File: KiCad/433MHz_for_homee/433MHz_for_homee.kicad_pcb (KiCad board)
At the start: 2 copper layers, 90 x 58.5 mm, 10 parts, among them Q1 BC547, Q2 BC547, SW1 SysMode, U1 ESP32-C3_SUPERMINI_TH, U2 4x Level Converter Module (3.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

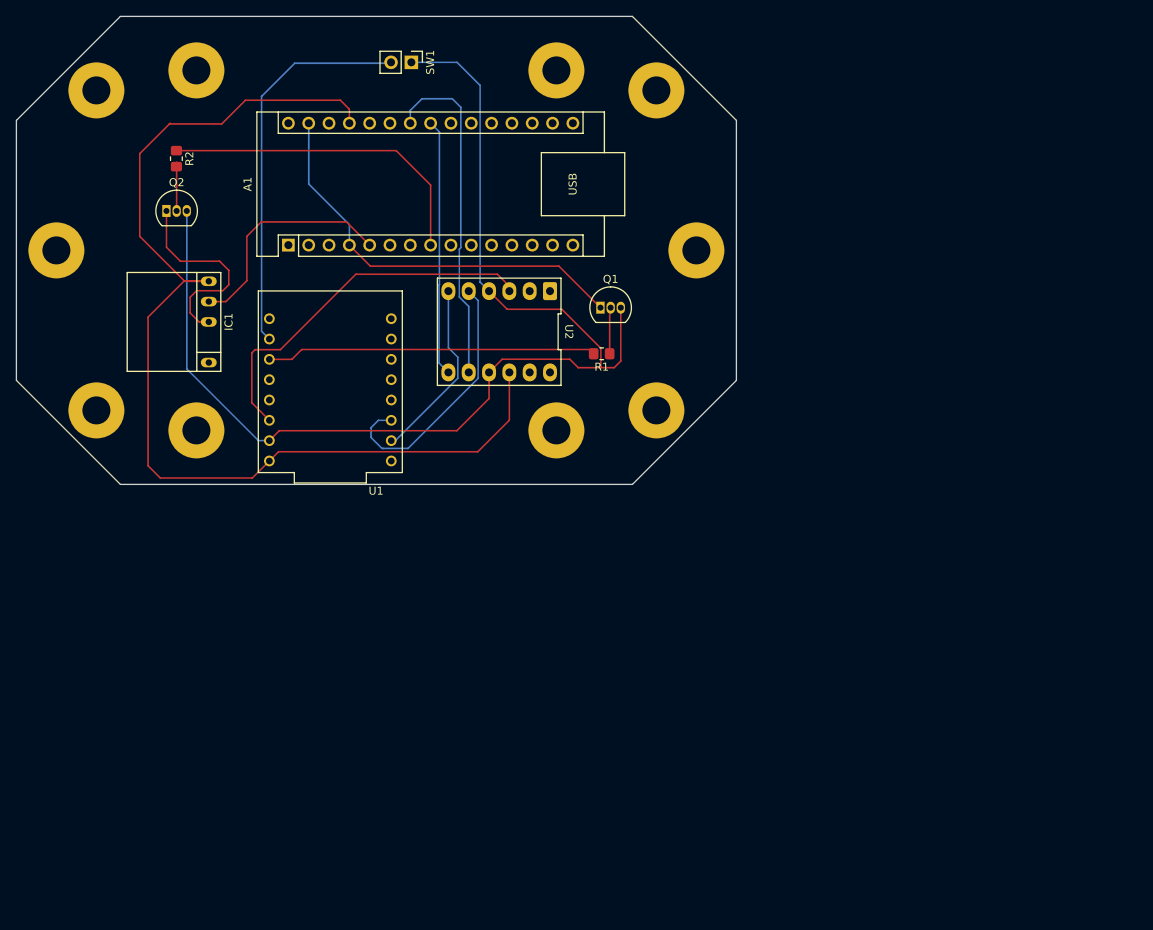
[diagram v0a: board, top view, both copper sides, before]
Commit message: User manual updated
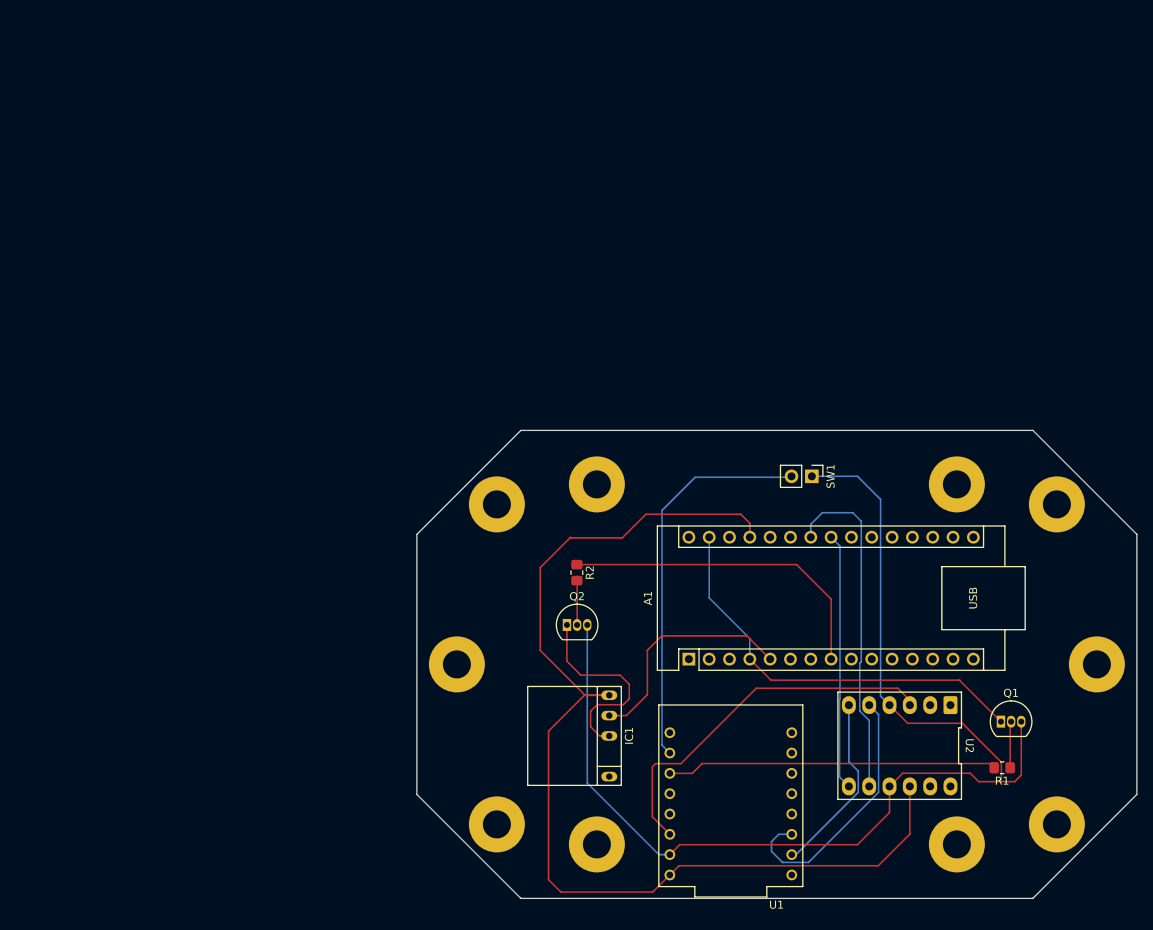
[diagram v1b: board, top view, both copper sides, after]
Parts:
- moved IC1 72.0 mm to (121.4, 113.4)
- moved U1 72.0 mm to (136.6, 120.9)
- moved A1 72.0 mm to (131.3, 103.8)
- moved Q1 72.0 mm to (170.3, 111.6)
- moved R1 72.0 mm to (170.5, 117.4)
- moved R2 72.0 mm to (117.3, 93.0)
- moved REF** 72.0 mm to (142.3, 104.5)
- moved SW1 72.0 mm to (146.7, 81.0)
- moved U2 72.0 mm to (157.7, 114.6)
- moved Q2 72.0 mm to (116.1, 99.5)
